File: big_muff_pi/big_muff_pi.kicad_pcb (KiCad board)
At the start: 2 copper layers, 80 x 100 mm, 78 parts, among them J1 Jack_6.35, J2 Jack_6.35, J6 top_panel_connector, J7 Conn_01x01_Socket, J8 Conn_01x01_Socket, J9 Barrel_Jack_Switch, P1 front_panel, P2 bottom_panel, Q1 MMBT5551, Q10 AO3401A, Q12 AO3400A, Q13 AO3400A, Q14 AO3400A, Q2 MMBT5551, Q3 MMBT5551, Q4 MMBT5551, Q5 MMBT5551, Q6 AO3401A, Q8 AO3401A, SW1 pedala_switch

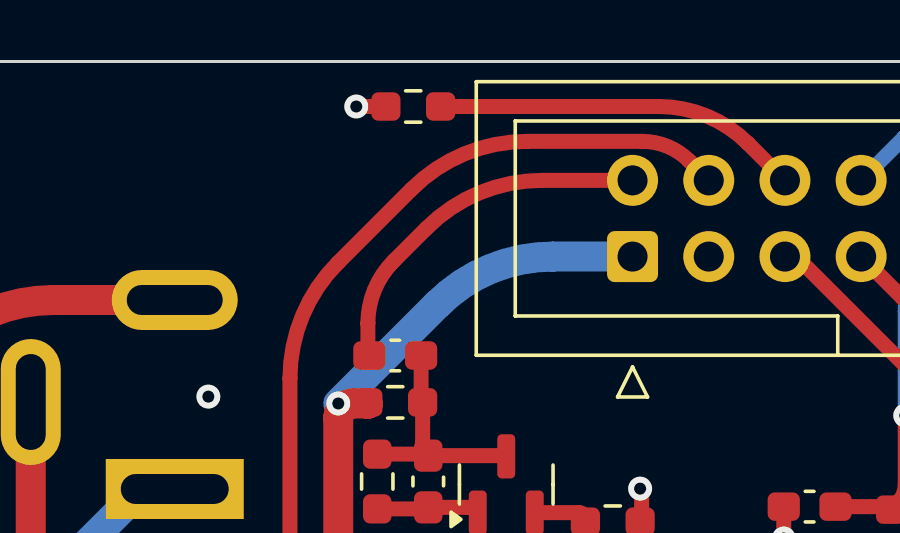
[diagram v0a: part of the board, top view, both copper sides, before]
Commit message: dfasdf dfasdf
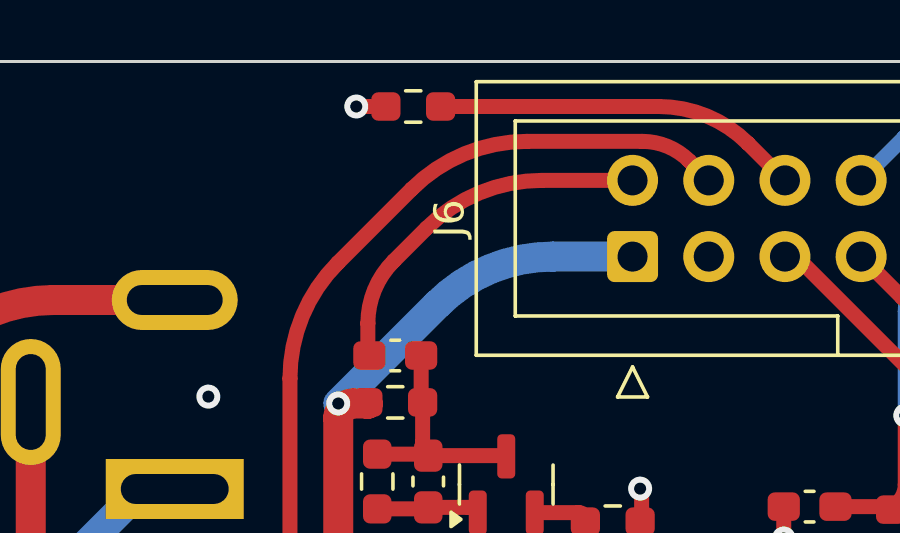
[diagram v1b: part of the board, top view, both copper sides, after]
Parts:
- J6: footprint Connector_IDC:IDC-Header_2x08_P2.54mm_Vertical -> pedale:IDC-Header_2x08_P2.54mm_Vertical
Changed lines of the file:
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@@
 		)
 	)
-	(footprint "Connector_IDC:IDC-Header_2x08_P2.54mm_Vertical"
+	(footprint "pedale:IDC-Header_2x08_P2.54mm_Vertical"
 		(locked yes)
 		(layer "F.Cu")
@@
 			(at 1.27 -6.1 90)
 			(layer "F.SilkS")
-			(hide yes)
 			(effects
 				(font
@@
 		)
 		(fp_text user "${REFERENCE}"
-			(at 1.27 8.89 0)
+			(at 1.27 8.89 180)
 			(layer "F.Fab")
 			(effects
@@
 			)
 		)
+		(model "${KIPRJMOD}/../pedale.pretty/IDC_female_16_no_strain.step"
+			(offset
+				(xyz 1.5 -8.9 9.5)
+			)
+			(scale
+				(xyz 1 1 1)
+			)
+			(rotate
+				(xyz -90 -0 -90)
+			)
+		)

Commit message: Production ready.
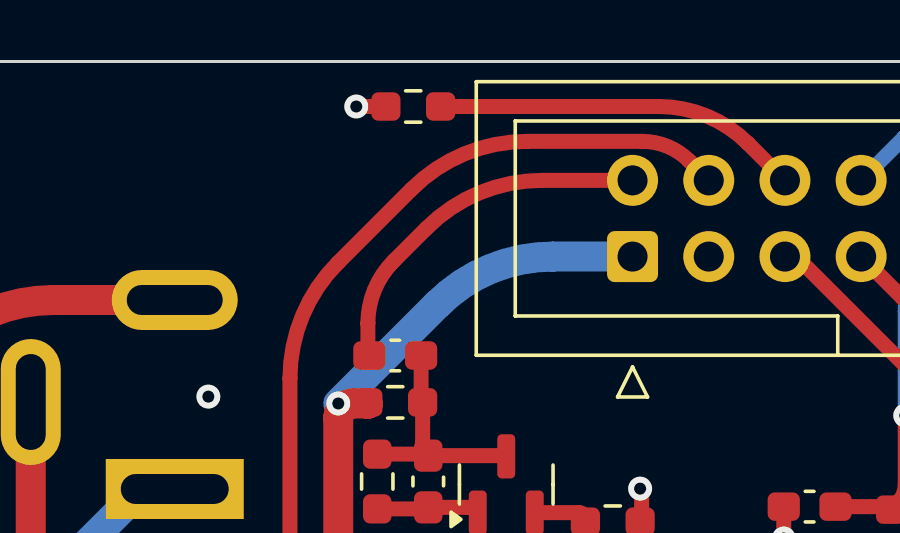
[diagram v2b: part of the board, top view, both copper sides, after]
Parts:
- removed D8: floating_green_led, pedale:floating_green_led
- removed D9: floating_red_led, pedale:floating_red_led
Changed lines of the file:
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@@
 		)
 	)
-	(footprint "pedale:floating_red_led"
-		(locked yes)
-		(layer "F.Cu")
-		(at 106 117)
-		(property "Reference" "D9"
-			(at 0 -0.5 0)
-			(unlocked yes)
-			(layer "F.SilkS")
-			(hide yes)
-			(effects
-				(font
-					(size 1 1)
-					(thickness 0.1)
-				)
-			)
-		)
-		(property "Value" "floating_red_led"
-			(at 0 1 0)
-			(unlocked yes)
-			(layer "F.Fab")
-			(effects
-				(font
-					(size 1 1)
-					(thickness 0.15)
-				)
-			)
-		)
-		(property "Datasheet" ""
-			(at 0 0 0)
-			(unlocked yes)
-			(layer "F.Fab")
-			(hide yes)
-			(effects
-				(font
-					(size 1 1)
-					(thickness 0.15)
-				)
-			)
-		)
-		(property "Description" "Light emitting diode"
-			(at 0 0 0)
-			(unlocked yes)
-			(layer "F.Fab")
-			(hide yes)
-			(effects
-				(font
-					(size 1 1)
-					(thickness 0.15)
-				)
-			)
-		)
-		(property "Sim.Pins" "1=K 2=A"
-			(at 0 0 0)
-			(unlocked yes)
-			(layer "F.Fab")
-			(hide yes)
-			(effects
-				(font
-					(size 1 1)
-					(thickness 0.15)
-				)
-			)
-		)
-		(property ki_fp_filters "LED* LED_SMD:* LED_THT:*")
-		(sheetname "/")
-		(sheetfile "big_muff_pi.kicad_sch")
-		(attr through_hole)
-		(fp_rect
-			(start -0.1 -0.1)
-			(end 0.1 0.1)
-			(stroke
-				(width 0.05)
-				(type default)
-			)
-			(fill no)
-			(layer "B.CrtYd")
-		)
-		(fp_text user "${REFERENCE}"
-			(at 0 2.5 0)
-			(unlocked yes)
-			(layer "F.Fab")
-			(effects
-				(font
-					(size 1 1)
-					(thickness 0.15)
-				)
-			)
-		)
-		(embedded_fonts no)
-		(model "${KIPRJMOD}/pedale.pretty/LED 3mm, Red, Thru-hole, Right Angle PCB 1.stp"
-			(offset
-				(xyz 0 -2 23.5)
-			)
-			(scale
-				(xyz 1 1 1)
-			)
-			(rotate
-				(xyz 90 -0 -0)
-			)
-		)
-	)
 	(footprint "Resistor_SMD:R_0603_1608Metric_Pad0.98x0.95mm_HandSolder"
 		(layer "F.Cu")
@@
 			(at 1.27 -6.1 90)
 			(layer "F.SilkS")
+			(hide yes)
 			(effects
 				(font
@@
 			)
 		)
-	)
-	(footprint "pedale:floating_green_led"
-		(locked yes)
-		(layer "F.Cu")
-		(at 74 117)
-		(property "Reference" "D8"
-			(at 0 -0.5 0)
-			(unlocked yes)
-			(layer "F.SilkS")
-			(hide yes)
-			(effects
-				(font
-					(size 1 1)
-					(thickness 0.1)
-				)
-			)
-		)
-		(property "Value" "floating_green_led"
-			(at 0 1 0)
-			(unlocked yes)
-			(layer "F.Fab")
-			(effects
-				(font
-					(size 1 1)
-					(thickness 0.15)
-				)
-			)
-		)
-		(property "Datasheet" ""
-			(at 0 0 0)
-			(unlocked yes)
-			(layer "F.Fab")
-			(hide yes)
-			(effects
-				(font
-					(size 1 1)
-					(thickness 0.15)
-				)
-			)
-		)
-		(property "Description" "Light emitting diode"
-			(at 0 0 0)
-			(unlocked yes)
-			(layer "F.Fab")
-			(hide yes)
-			(effects
-				(font
-					(size 1 1)
-					(thickness 0.15)
-				)
-			)
-		)
-		(property "Sim.Pins" "1=K 2=A"
-			(at 0 0 0)
-			(unlocked yes)
-			(layer "F.Fab")
-			(hide yes)
-			(effects
-				(font
-					(size 1 1)
-					(thickness 0.15)
-				)
-			)
-		)
-		(property ki_fp_filters "LED* LED_SMD:* LED_THT:*")
-		(sheetname "/")
-		(sheetfile "big_muff_pi.kicad_sch")
-		(attr through_hole)
-		(fp_rect
-			(start -0.1 -0.1)
-			(end 0.1 0.1)
-			(stroke
-				(width 0.05)
-				(type default)
-			)
-			(fill no)
-			(layer "B.CrtYd")
-		)
-		(fp_text user "${REFERENCE}"
-			(at 0 2.5 0)
-			(unlocked yes)
-			(layer "F.Fab")
-			(effects
-				(font
-					(size 1 1)
-					(thickness 0.15)
-				)
-			)
-		)
-		(embedded_fonts no)
-		(model "${KIPRJMOD}/pedale.pretty/LED 3mm, Green, Thru-hole, Right Angle PCB 1.stp"
-			(offset
-				(xyz 0 -2 23.5)
-			)
-			(scale
-				(xyz 1 1 1)
-			)
-			(rotate
-				(xyz 90 -0 -0)
-			)
-		)
